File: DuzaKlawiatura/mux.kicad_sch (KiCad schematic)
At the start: 25 parts, among them U1 CD74HC4067SM, U2 CD74HC4067SM, U3 CD74HC4067SM, U4 CD74HC4067SM, U5 CD74HC4067SM

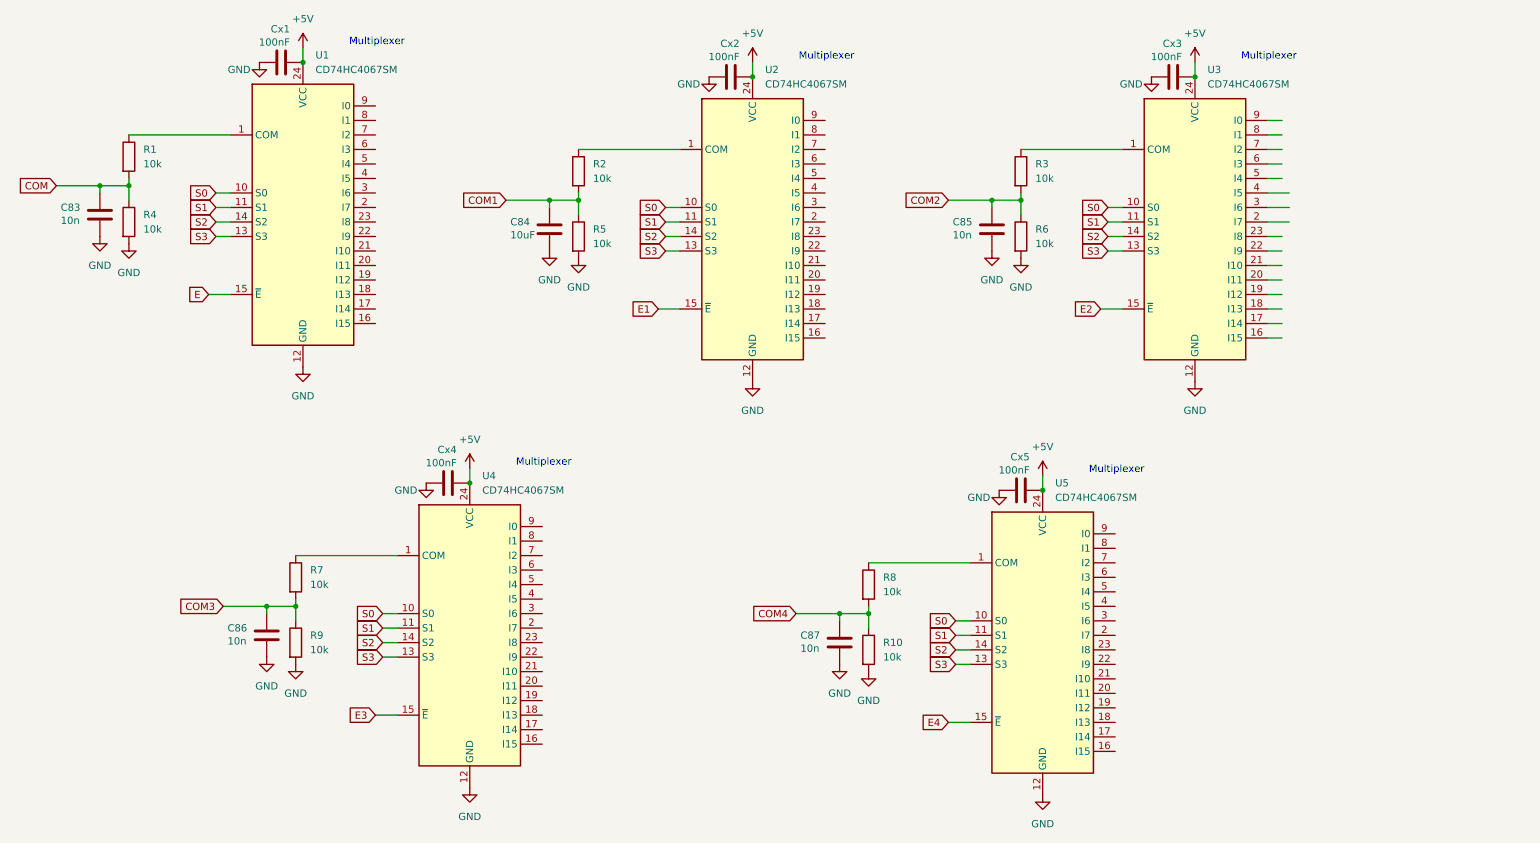
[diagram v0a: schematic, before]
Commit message: Added photos of layout and schematic, updated Kicad files.
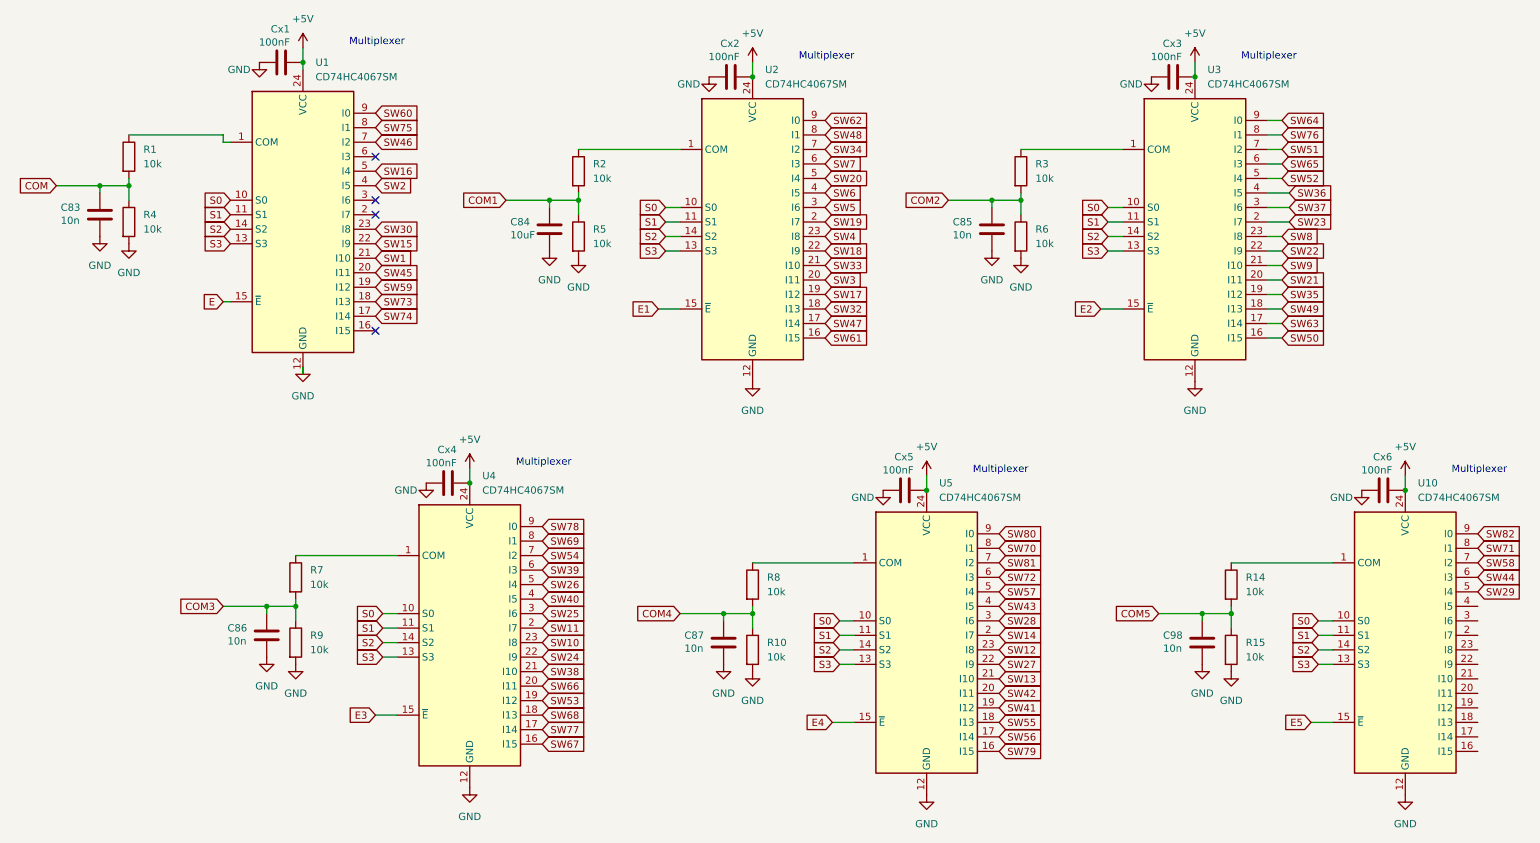
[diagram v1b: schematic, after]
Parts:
- added C98: 10n, Capacitor_SMD:C_0402_1005Metric, symbol Device:C
- added Cx6: 100nF, Capacitor_SMD:C_0402_1005Metric, symbol Device:C
- added R14, R15: 10k, Resistor_SMD:R_0402_1005Metric, symbol Device:R
- added U10: CD74HC4067SM, Package_SO:SSOP-24_5.3x8.2mm_P0.65mm, symbol 74xx:CD74HC4067SM
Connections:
- net +5V: now also Cx6.2, U10.24 (VCC)
- net GND: now also C98.2, Cx6.1, R15.2, U10.12 (GND)
- net S0: now also U10.10 (S0)
- net S1: now also U10.11 (S1)
- net S2: now also U10.14 (S2)
- net S3: now also U10.13 (S3)
- net SW67: now reaches U4.16 (I15)
- net SW77: now reaches U4.17 (I14)
- net SW68: now reaches U4.18 (I13)
- net SW53: now reaches U4.19 (I12)
- net SW11: now reaches U4.2 (I7)
- net SW66: now reaches U4.20 (I11)
- net SW38: now reaches U4.21 (I10)
- net SW24: now reaches U4.22 (I9)
- net SW10: now reaches U4.23 (I8)
- net SW25: now reaches U4.3 (I6)
- net SW40: now reaches U4.4 (I5)
- net SW26: now reaches U4.5 (I4)
- net SW39: now reaches U4.6 (I3)
- net SW54: now reaches U4.7 (I2)
- net SW69: now reaches U4.8 (I1)
- net SW78: now reaches U4.9 (I0)
- net SW74: now reaches U1.17 (I14)
- net SW73: now reaches U1.18 (I13)
- net SW59: now reaches U1.19 (I12)
- net SW45: now reaches U1.20 (I11)
- net SW1: now reaches U1.21 (I10)
- net SW15: now reaches U1.22 (I9)
- net SW30: now reaches U1.23 (I8)
- net SW2: now reaches U1.4 (I5)
- net SW16: now reaches U1.5 (I4)
- net SW46: now reaches U1.7 (I2)
- net SW75: now reaches U1.8 (I1)
- net SW60: now reaches U1.9 (I0)
- net SW50: now reaches U3.16 (I15)
- net SW63: now reaches U3.17 (I14)
- net SW49: now reaches U3.18 (I13)
- net SW35: now reaches U3.19 (I12)
- net SW23: now reaches U3.2 (I7)
- net SW21: now reaches U3.20 (I11)
- net SW9: now reaches U3.21 (I10)
- net SW22: now reaches U3.22 (I9)
- net SW8: now reaches U3.23 (I8)
- net SW37: now reaches U3.3 (I6)
- net SW36: now reaches U3.4 (I5)
- net SW52: now reaches U3.5 (I4)
- net SW65: now reaches U3.6 (I3)
- net SW51: now reaches U3.7 (I2)
- net SW76: now reaches U3.8 (I1)
- net SW64: now reaches U3.9 (I0)
- net SW61: now reaches U2.16 (I15)
- net SW47: now reaches U2.17 (I14)
- net SW32: now reaches U2.18 (I13)
- net SW17: now reaches U2.19 (I12)
- net SW19: now reaches U2.2 (I7)
- net SW3: now reaches U2.20 (I11)
- net SW33: now reaches U2.21 (I10)
- net SW18: now reaches U2.22 (I9)
- net SW4: now reaches U2.23 (I8)
- net SW5: now reaches U2.3 (I6)
- net SW6: now reaches U2.4 (I5)
- net SW20: now reaches U2.5 (I4)
- net SW7: now reaches U2.6 (I3)
- net SW34: now reaches U2.7 (I2)
- net SW48: now reaches U2.8 (I1)
- net SW62: now reaches U2.9 (I0)
- net SW79: now reaches U5.16 (I15)
- net SW56: now reaches U5.17 (I14)
- net SW55: now reaches U5.18 (I13)
- net SW41: now reaches U5.19 (I12)
- net SW14: now reaches U5.2 (I7)
- net SW42: now reaches U5.20 (I11)
- net SW13: now reaches U5.21 (I10)
- net SW27: now reaches U5.22 (I9)
- net SW12: now reaches U5.23 (I8)
- net SW28: now reaches U5.3 (I6)
- net SW43: now reaches U5.4 (I5)
- net SW57: now reaches U5.5 (I4)
- net SW72: now reaches U5.6 (I3)
- net SW81: now reaches U5.7 (I2)
- net SW70: now reaches U5.8 (I1)
- net SW80: now reaches U5.9 (I0)
- new net: R14.1, U10.1 (COM)
- new net COM5: C98.1, R14.2, R15.1
- new net E5: U10.15 (~{E})
- new net SW29: U10.5 (I4)
- new net SW44: U10.6 (I3)
- new net SW58: U10.7 (I2)
- new net SW71: U10.8 (I1)
- new net SW82: U10.9 (I0)
- no-connect marks 0 -> 4
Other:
- moved on the sheet: C87, Cx5, R10, R8, U1, U5
